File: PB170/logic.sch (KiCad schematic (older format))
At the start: 0 parts

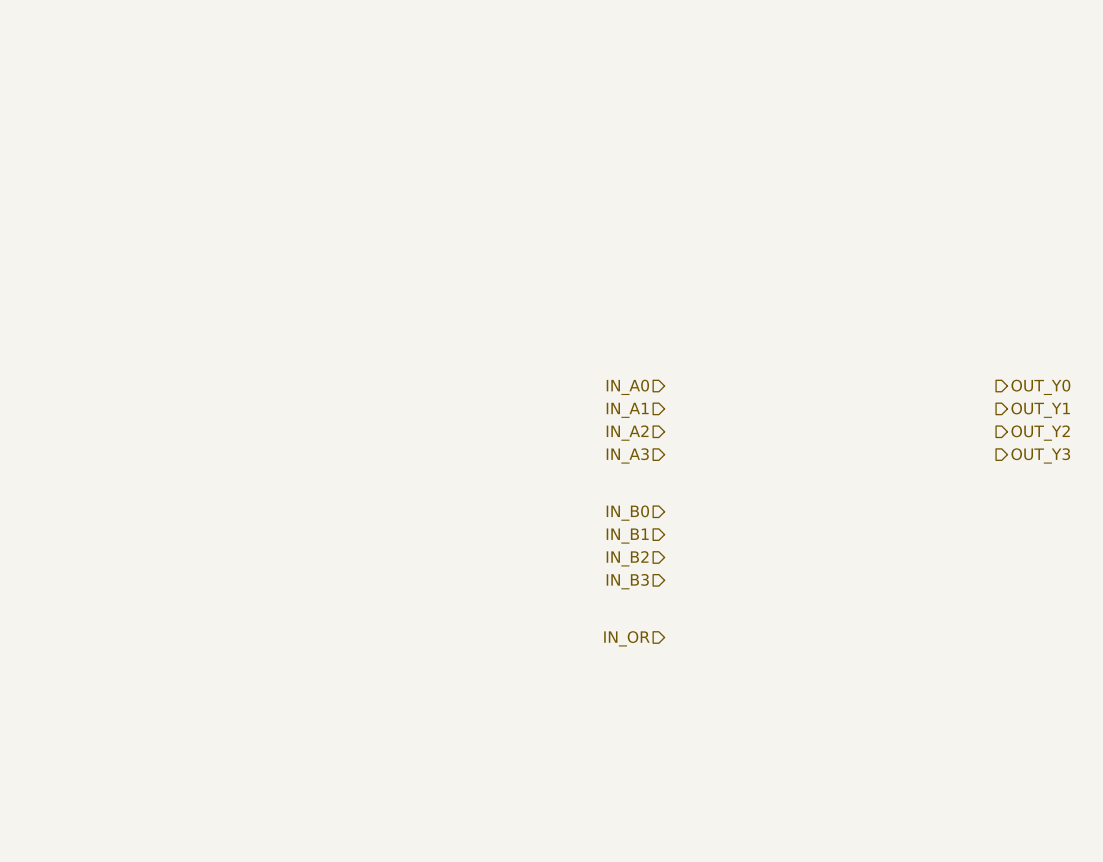
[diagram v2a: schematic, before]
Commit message: ALU finished
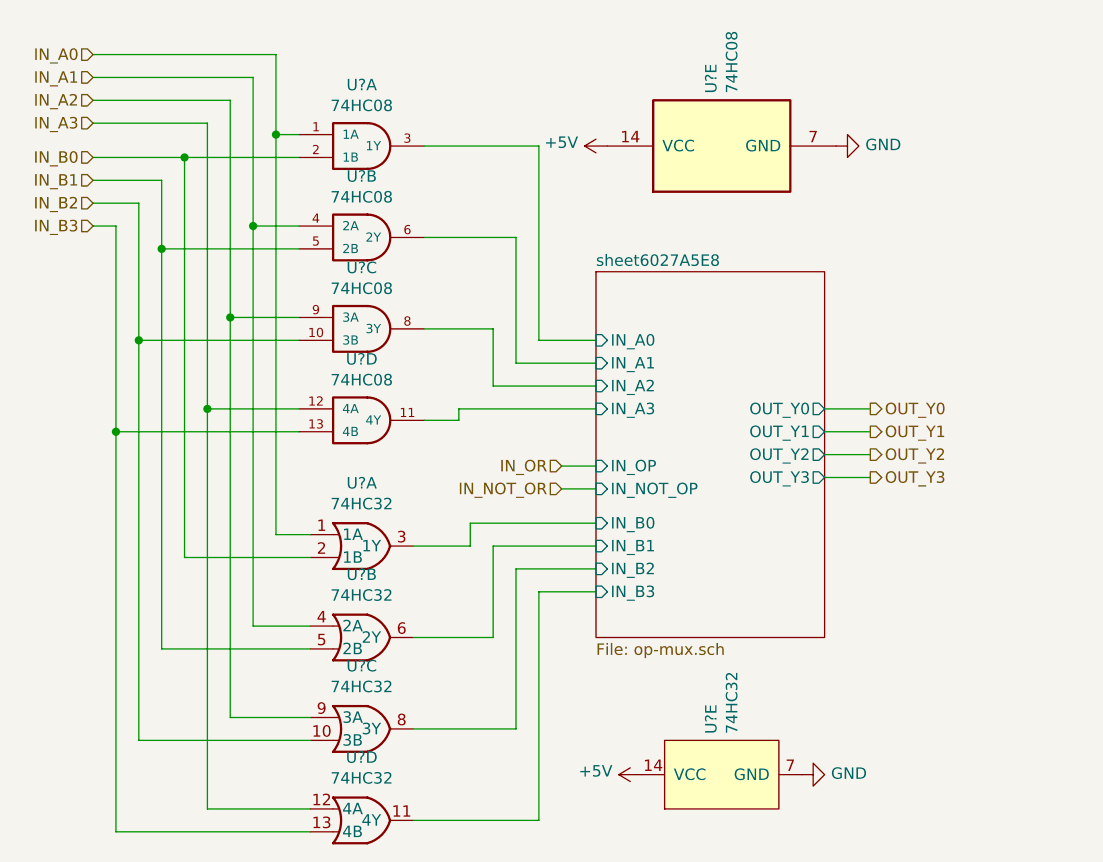
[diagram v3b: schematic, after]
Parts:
- added U? (x5): 74HC32, Housings_SOIC:SOIC-14_3.9x8.7mm_Pitch1.27mm, symbol PB170:74HC32
- added U? (x5): 74HC08, Housings_SOIC:SOIC-14_3.9x8.7mm_Pitch1.27mm, symbol PB170:74HC08
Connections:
- net IN_A0: now also U?.1 (1A), U?.1 (1A)
- net IN_A1: now also U?.4 (2A), U?.4 (2A)
- net IN_A2: now also U?.9 (3A), U?.9 (3A)
- net IN_A3: now also U?.12 (4A), U?.12 (4A)
- net IN_B0: now also U?.2 (1B), U?.2 (1B)
- net IN_B1: now also U?.5 (2B), U?.5 (2B)
- net IN_B2: now also U?.10 (3B), U?.10 (3B)
- net IN_B3: now also U?.13 (4B), U?.13 (4B)
- new net +5V: U?.14 (VCC), U?.14 (VCC)
- new net GND: U?.7 (GND), U?.7 (GND)
- new net sheet6027A5E8/IN_A0: U?.3 (1Y)
- new net sheet6027A5E8/IN_A1: U?.6 (2Y)
- new net sheet6027A5E8/IN_A2: U?.8 (3Y)
- new net sheet6027A5E8/IN_A3: U?.11 (4Y)
- new net sheet6027A5E8/IN_B0: U?.3 (1Y)
- new net sheet6027A5E8/IN_B1: U?.6 (2Y)
- new net sheet6027A5E8/IN_B2: U?.8 (3Y)
- new net sheet6027A5E8/IN_B3: U?.11 (4Y)
